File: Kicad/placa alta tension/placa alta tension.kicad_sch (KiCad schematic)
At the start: 32 parts, among them J1 Conn_01x05_Socket, J2 Screw_Terminal_01x02, J3 Screw_Terminal_01x02, J4 Screw_Terminal_01x02, Q2 2N7000, Q4 2N7000, U1 MOC3023M, U2 4N25, U3 MOC3023M

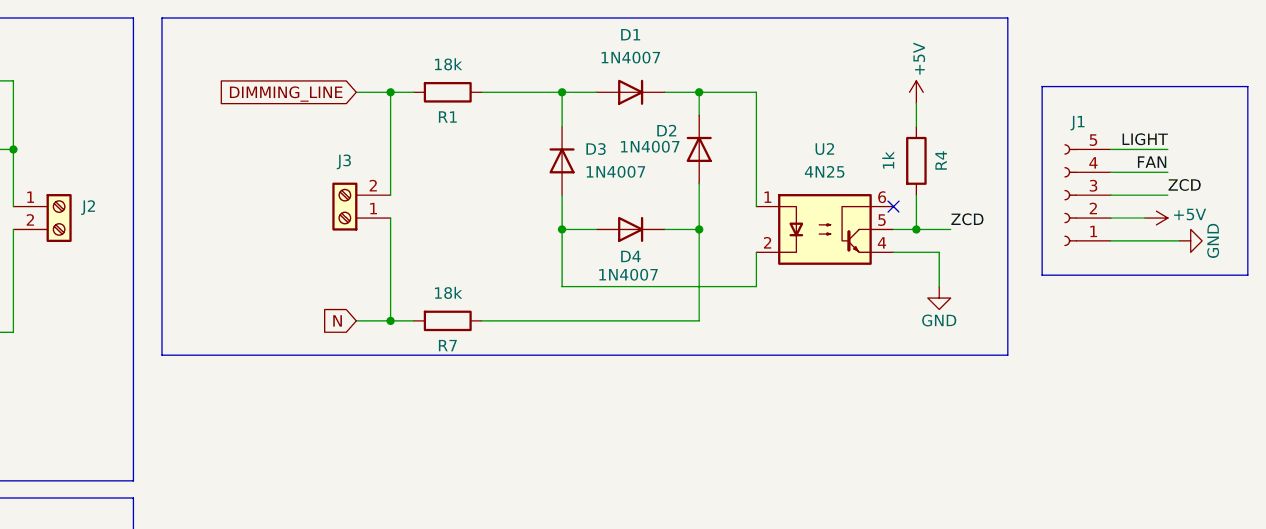
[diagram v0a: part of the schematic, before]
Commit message: consulta Fede
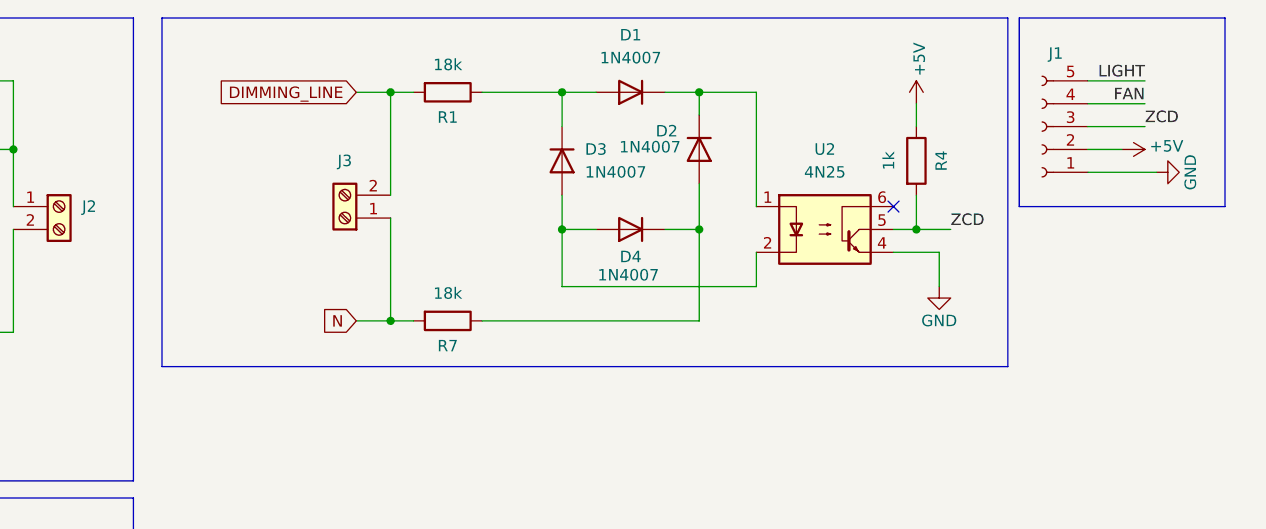
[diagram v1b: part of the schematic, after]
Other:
- moved on the sheet: J1
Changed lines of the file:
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@@
 	(rectangle
 		(start 124.46 14.605)
-		(end 218.44 52.07)
+		(end 218.44 53.34)
 		(stroke
 			(width 0)
@@
 	)
 	(rectangle
-		(start 222.25 22.225)
-		(end 245.11 43.18)
+		(start 219.71 14.605)
+		(end 242.57 35.56)
 		(stroke
 			(width 0)
@@
 	(wire
 		(pts
-			(xy 236.22 34.29) (xy 229.87 34.29)
+			(xy 233.68 26.67) (xy 227.33 26.67)
 		)
 		(stroke
@@
 	(wire
 		(pts
-			(xy 237.49 39.37) (xy 229.87 39.37)
+			(xy 234.95 31.75) (xy 227.33 31.75)
 		)
 		(stroke
@@
 	(wire
 		(pts
-			(xy 229.87 36.83) (xy 233.68 36.83)
+			(xy 227.33 29.21) (xy 231.14 29.21)
 		)
 		(stroke
@@
 	(wire
 		(pts
-			(xy 236.22 31.75) (xy 229.87 31.75)
+			(xy 233.68 24.13) (xy 227.33 24.13)
 		)
 		(stroke
@@
 	(wire
 		(pts
-			(xy 236.22 29.21) (xy 229.87 29.21)
+			(xy 233.68 21.59) (xy 227.33 21.59)
 		)
 		(stroke
@@
 	)
 	(label "LIGHT"
-		(at 236.22 29.21 180)
+		(at 233.68 21.59 180)
 		(effects
 			(font
@@
 	)
 	(label "ZCD"
-		(at 236.22 34.29 0)
+		(at 233.68 26.67 0)
 		(effects
 			(font
@@
 	)
 	(label "FAN"
-		(at 236.22 31.75 180)
+		(at 233.68 24.13 180)
 		(effects
 			(font
@@
 	(symbol
 		(lib_id "Connector:Conn_01x05_Socket")
-		(at 224.79 34.29 180)
+		(at 222.25 26.67 180)
 		(unit 1)
 		(exclude_from_sim no)
@@
 		(dnp no)
 		(property "Reference" "J1"
-			(at 226.314 26.162 0)
+			(at 223.774 18.542 0)
 			(effects
 				(font
@@
 		)
 		(property "Value" "Conn_01x05_Socket"
-			(at 225.425 26.67 0)
+			(at 222.885 19.05 0)
 			(effects
 				(font
@@
 		)
 		(property "Footprint" "Connector_PinHeader_2.54mm:PinHeader_1x05_P2.54mm_Horizontal"
-			(at 224.79 34.29 0)
+			(at 222.25 26.67 0)
 			(effects
 				(font
@@
 		)
 		(property "Datasheet" "~"
-			(at 224.79 34.29 0)
+			(at 222.25 26.67 0)
 			(effects
 				(font
@@
 		)
 		(property "Description" "Generic connector, single row, 01x05, script generated"
-			(at 224.79 34.29 0)
+			(at 222.25 26.67 0)
 			(effects
 				(font
@@
 	(symbol
 		(lib_id "power:GND")
-		(at 237.49 39.37 90)
+		(at 234.95 31.75 90)
 		(mirror x)
 		(unit 1)
@@
 		(dnp no)
 		(property "Reference" "#PWR04"
-			(at 243.84 39.37 0)
+			(at 241.3 31.75 0)
 			(effects
 				(font
@@
 		)
 		(property "Value" "GND"
-			(at 241.3 39.37 0)
+			(at 238.76 31.75 0)
 			(effects
 				(font
@@
 		)
 		(property "Footprint" ""
-			(at 237.49 39.37 0)
+			(at 234.95 31.75 0)
 			(effects
 				(font
@@
 		)
 		(property "Datasheet" ""
-			(at 237.49 39.37 0)
+			(at 234.95 31.75 0)
 			(effects
 				(font
@@
 		)
 		(property "Description" "Power symbol creates a global label with name \"GND\" , ground"
-			(at 237.49 39.37 0)
+			(at 234.95 31.75 0)
 			(effects
 				(font
@@
 	(symbol
 		(lib_id "power:+5V")
-		(at 233.68 36.83 270)
+		(at 231.14 29.21 270)
 		(mirror x)
 		(unit 1)
@@
 		(dnp no)
 		(property "Reference" "#PWR03"
-			(at 229.87 36.83 0)
+			(at 227.33 29.21 0)
 			(effects
 				(font
@@
 		)
 		(property "Value" "+5V"
-			(at 236.728 36.4744 90)
+			(at 234.188 28.8544 90)
 			(effects
 				(font
@@
 		)
 		(property "Footprint" ""
-			(at 233.68 36.83 0)
+			(at 231.14 29.21 0)
 			(effects
 				(font
@@
 		)
 		(property "Datasheet" ""
-			(at 233.68 36.83 0)
+			(at 231.14 29.21 0)
 			(effects
 				(font
@@
 		)
 		(property "Description" "Power symbol creates a global label with name \"+5V\""
-			(at 233.68 36.83 0)
+			(at 231.14 29.21 0)
 			(effects
 				(font
